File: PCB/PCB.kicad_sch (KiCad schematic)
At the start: 41 parts, among them J1 Conn_01x02, J2 Conn_01x02, J3 Conn_01x03, U1 Seeed Studio XIAO nRF52840, U2 Seeed Studio XIAO nRF52840

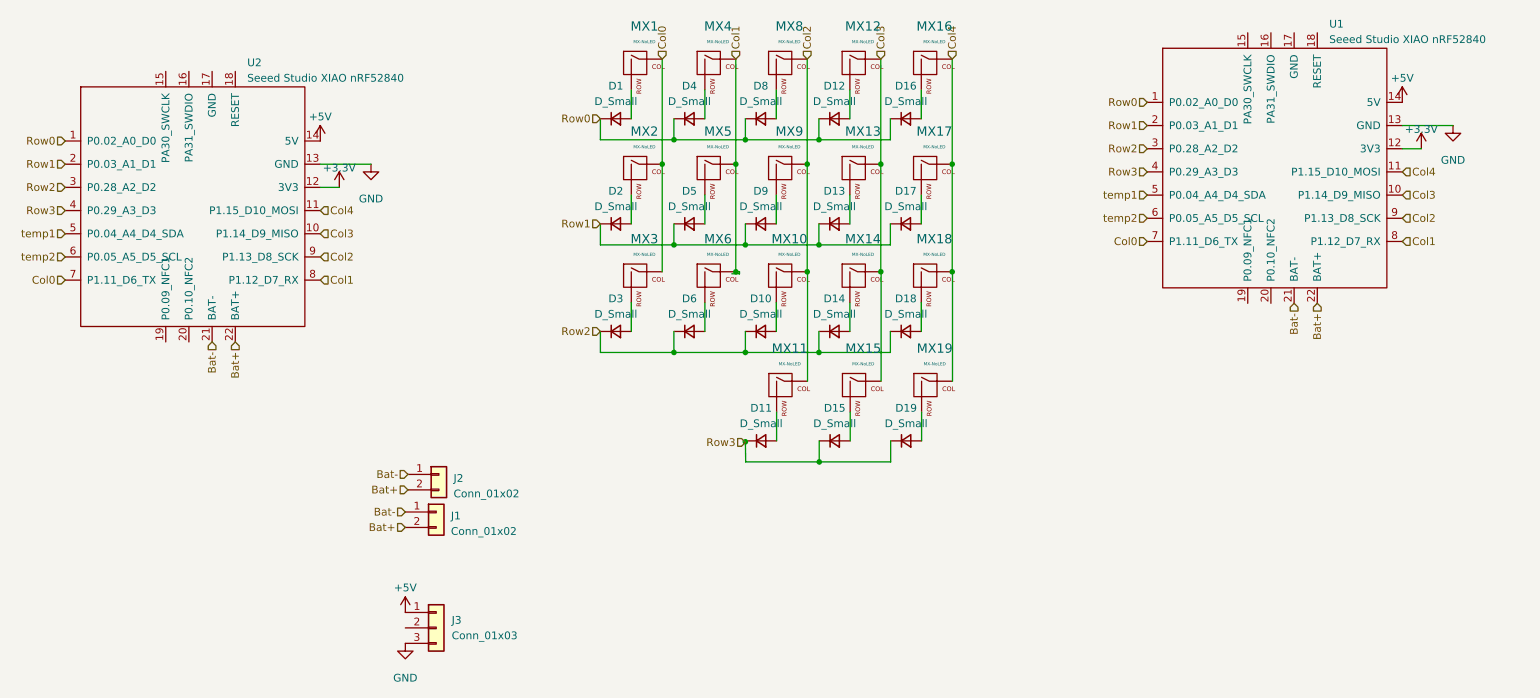
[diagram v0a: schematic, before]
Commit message: pcb v0.1
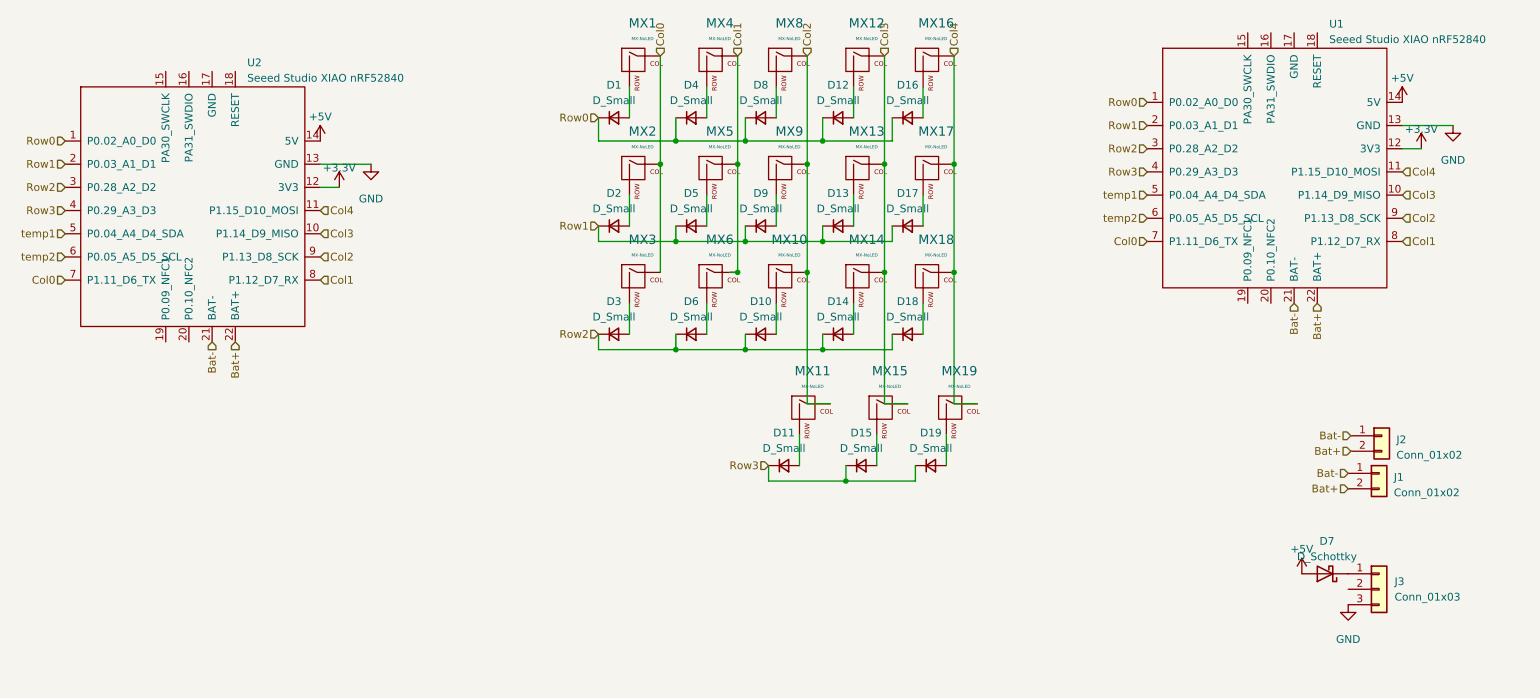
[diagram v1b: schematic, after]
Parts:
- added D7: D_Schottky, Diode_SMD:D_SMA, symbol Device:D_Schottky
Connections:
- net +5V: now also D7.2 (A); no longer J3.1 (Pin_1)
- new net: D7.1 (K), J3.1 (Pin_1)
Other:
- moved on the sheet: D11, D12, D13, D14, D15, D18, D19, D3, D6, J1, J2, J3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
